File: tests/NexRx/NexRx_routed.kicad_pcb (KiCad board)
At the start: 3 copper layers, 349 parts

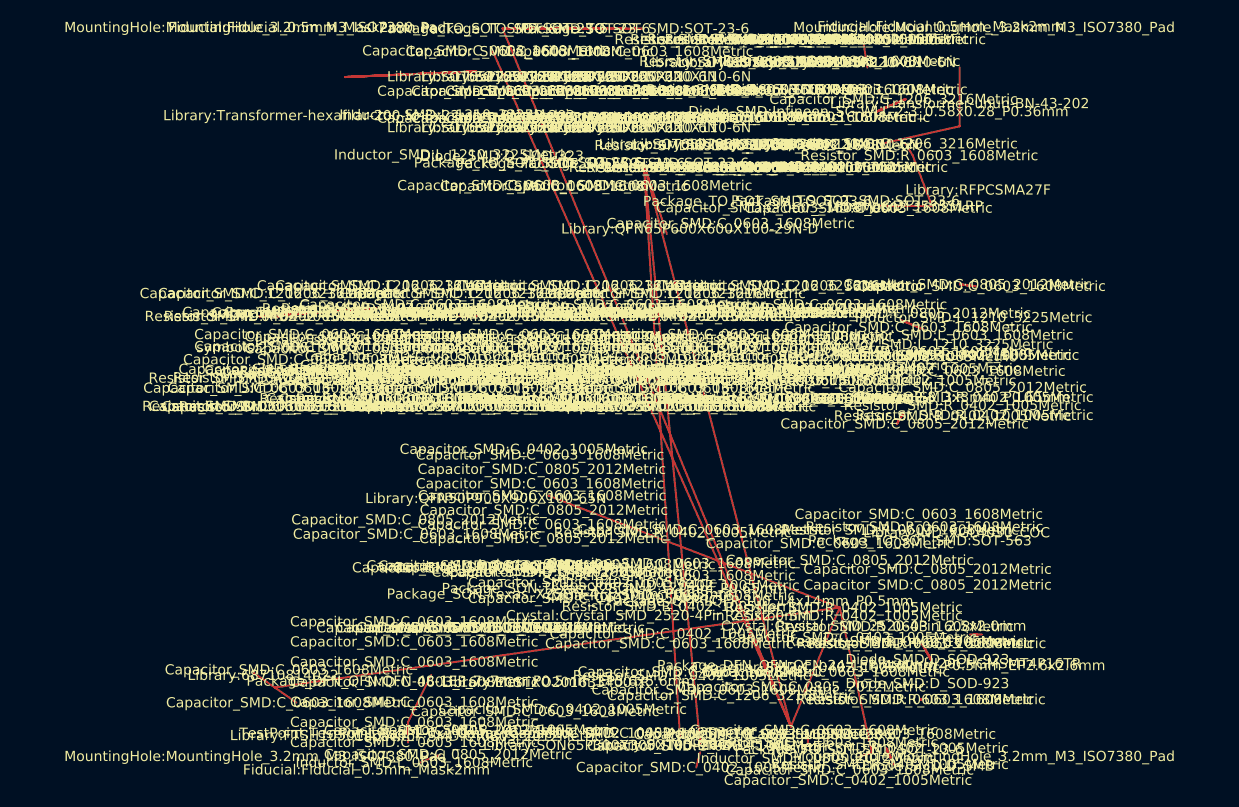
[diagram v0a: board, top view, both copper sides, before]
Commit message: Merge sanity pad size
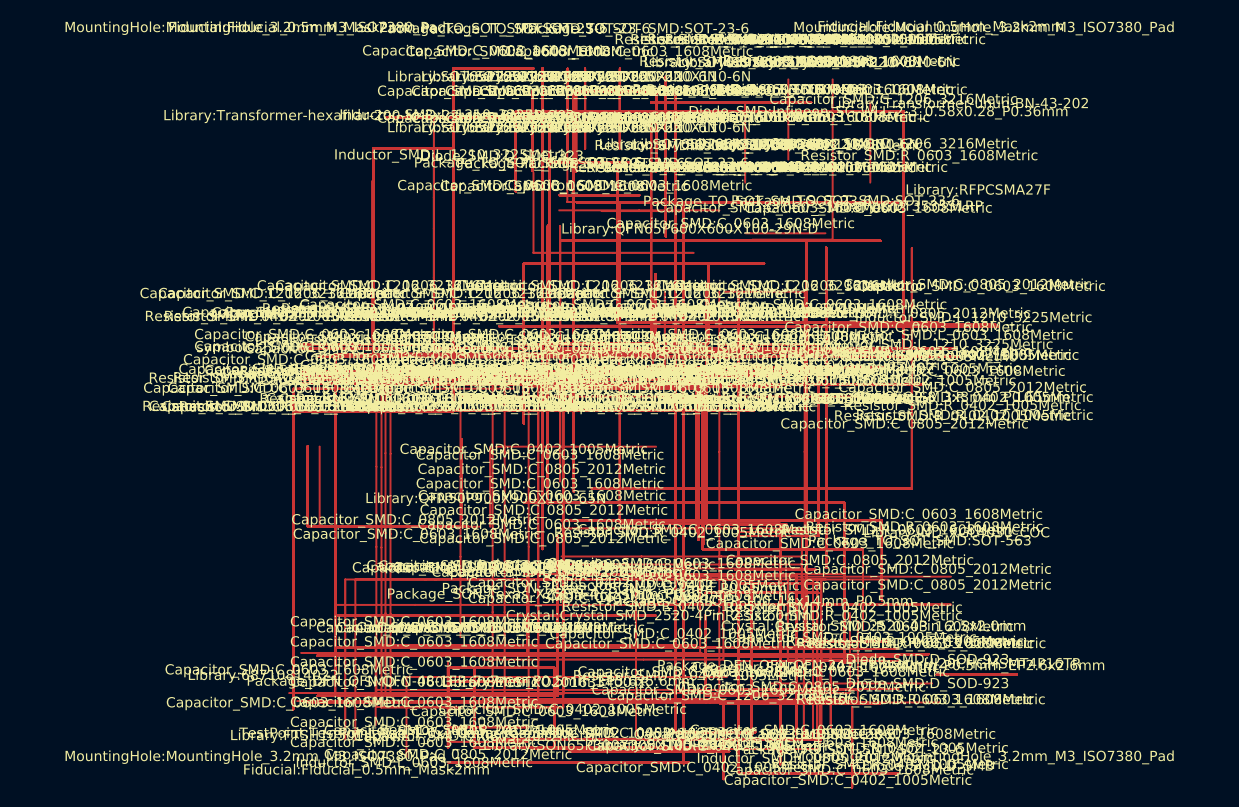
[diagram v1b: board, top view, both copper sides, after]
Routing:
- net +3.3V: track 599.8 -> 17100.0 mm
- net +2V5bias: track 54.3 -> 4200.0 mm
- net /Rx Front End/Rx Preselector/preselIn: track 65.4 -> 3700.0 mm
- net +1V65bias: track 7.29 -> 2320.0 mm
- net +3.3VFPGAIO: track 14.3 -> 2200.0 mm
- net +3.3V-ON: track 0.76 -> 2000.0 mm
- net /FPGA/Ctrl.qsdSCK: track 0.00 -> 1600.0 mm
- net /FPGA/Ctrl.qsdMOSI: track 0.00 -> 1600.0 mm
- net /FPGA/Ctrl.qsdNSS: track 0.00 -> 1500.0 mm
- net /FPGA/FPGA.NSS: track 0.00 -> 1000.0 mm
- net /FPGA/FPGA.SCK: track 0.00 -> 600.0 mm
- net nRESET: track 0.00 -> 510.0 mm
- net /FPGA/Ctrl.audioSCL: track 0.00 -> 500.0 mm
- net /Rx Front End/rxQ2-: track 0.00 -> 300.0 mm
- net +VFPGACORE: track 0.00 -> 300.0 mm
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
